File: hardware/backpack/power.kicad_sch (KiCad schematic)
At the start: 14 parts, among them J6 CONN 2x5 P=2.54mm, U5 AP63200WU

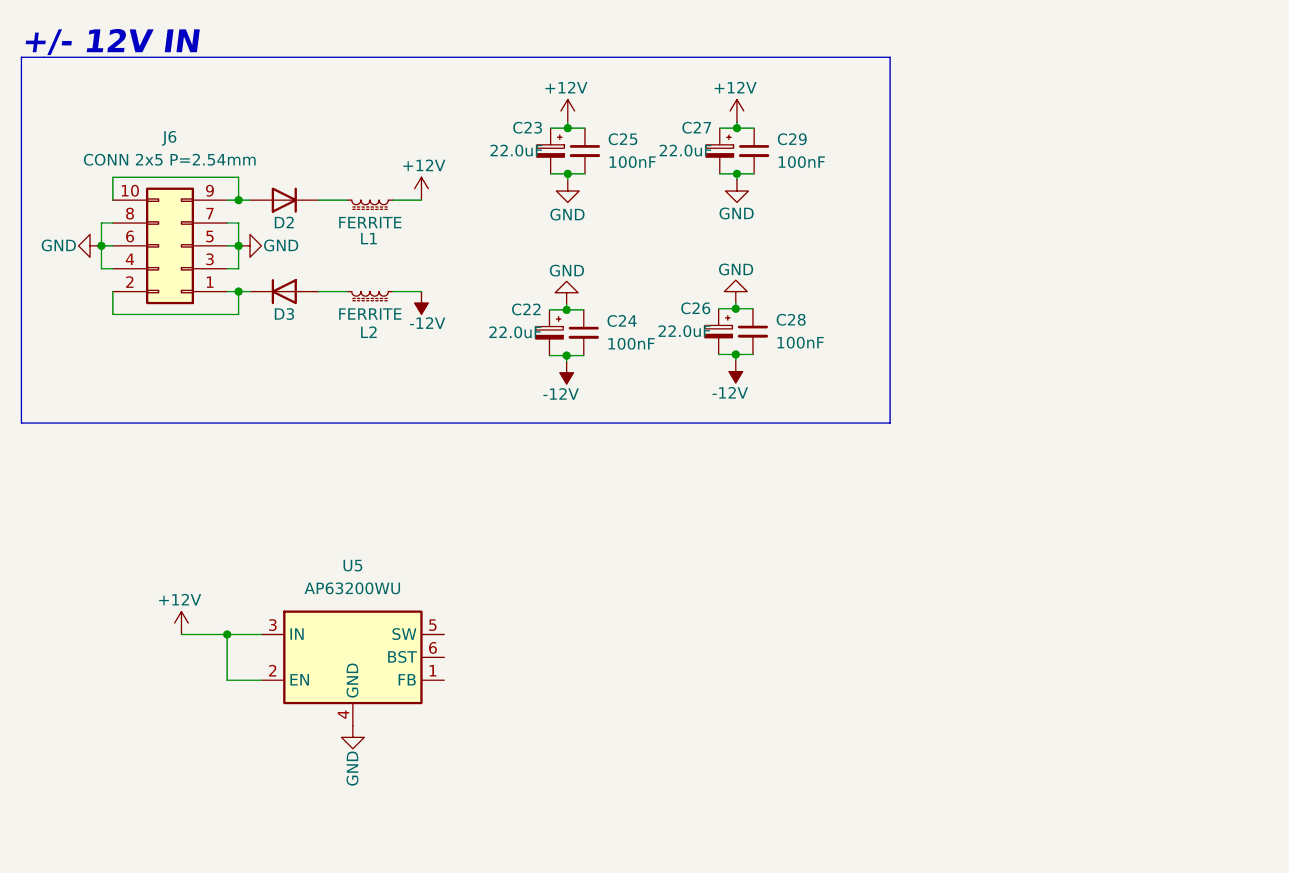
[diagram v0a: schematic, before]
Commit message: start on regs
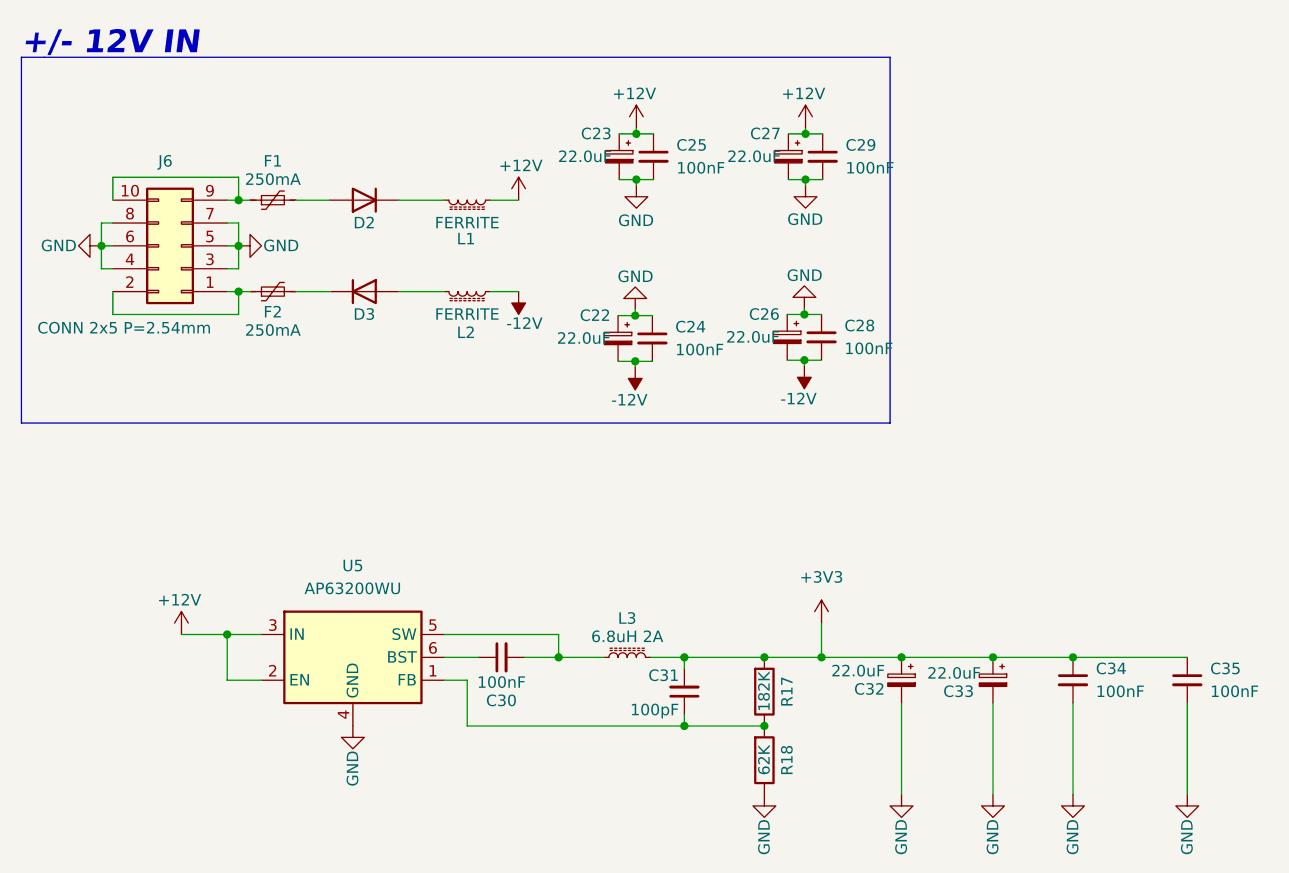
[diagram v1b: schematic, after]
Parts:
- added C30, C34, C35: 100nF, Capacitor_SMD:C_0603_1608Metric, symbol Device:C_Small
- added C31: 100pF, Capacitor_SMD:C_0603_1608Metric, symbol Device:C_Small
- added C32, C33: 22.0uF, Capacitor_Tantalum_SMD:CP_EIA-3216-10_Kemet-I, symbol Device:C_Polarized_Small
- added F1, F2: 250mA, symbol Device:Polyfuse_Small
- added L3: 6.8uH 2A, symbol Device:L_Ferrite_Small
- added R17: 182K, Resistor_SMD:R_0402_1005Metric, symbol Device:R
- added R18: 62K, Resistor_SMD:R_0402_1005Metric, symbol Device:R
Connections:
- net GND: now also C32.2, C33.2, C34.2, C35.2, R18.1
- net at J6.1 (Pin_1), J6.2 (Pin_2): now also F2.1; no longer D3.1 (K)
- net at J6.10 (Pin_10), J6.9 (Pin_9): now also F1.1; no longer D2.2 (A)
- net at U5.1 (FB): now also C31.1, R17.1, R18.2
- net at U5.5 (SW): now also C30.2, L3.1
- net at U5.6 (BST): now also C30.1
- new net: D3.1 (K), F2.2
- new net: D2.2 (A), F1.2
- new net +3V3: C31.2, C32.1, C33.1, C34.1, C35.1, L3.2, R17.2
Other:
- moved on the sheet: C22, C23, C24, C25, C26, C27, C28, C29, D2, D3, L1, L2
